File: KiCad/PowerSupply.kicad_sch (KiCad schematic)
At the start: 15 parts, among them U601 TPS54302, U602 MCP1825S

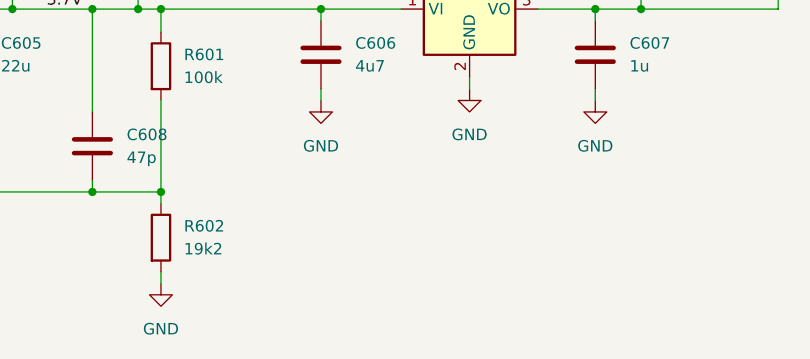
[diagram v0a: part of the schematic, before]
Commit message: KiCad work
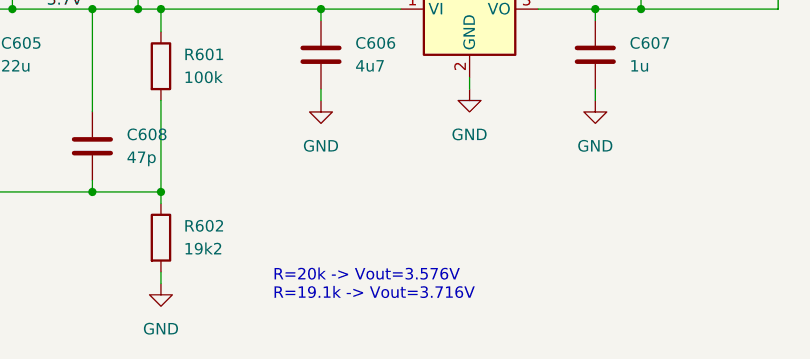
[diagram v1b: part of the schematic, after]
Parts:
- C601: footprint Capacitor_SMD:C_0201_0603Metric -> Capacitor_SMD:C_0805_2012Metric
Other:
- note added: "R=20k -> Vout=3.576V R=19.1k -> Vout=3.716V"
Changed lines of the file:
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@@
 	(generator_version "9.0")
 	(paper "A4")
+	(text "R=20k -> Vout=3.576V\nR=19.1k -> Vout=3.716V"
+		(exclude_from_sim no)
+		(at 186.436 122.936 0)
+		(effects
+			(font
+				(size 1.27 1.27)
+			)
+			(justify left top)
+		)
+	)
 	(junction
 		(at 173.99 93.98)
@@
 			)
 		)
-		(property "Footprint" "Capacitor_SMD:C_0201_0603Metric"
+		(property "Footprint" "Capacitor_SMD:C_0805_2012Metric"
 			(at 121.6152 91.44 0)
 			(effects
